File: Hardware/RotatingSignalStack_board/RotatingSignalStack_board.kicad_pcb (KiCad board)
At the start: 2 copper layers, 69.1 x 69 mm, 32 parts, among them J1 8P8C_LED_Shielded, J2 Conn_01x05_Pin, SW1 SW_Push, SW2 SW_Push, U1 OKI, U3 Teensy4.1_DEV-16771

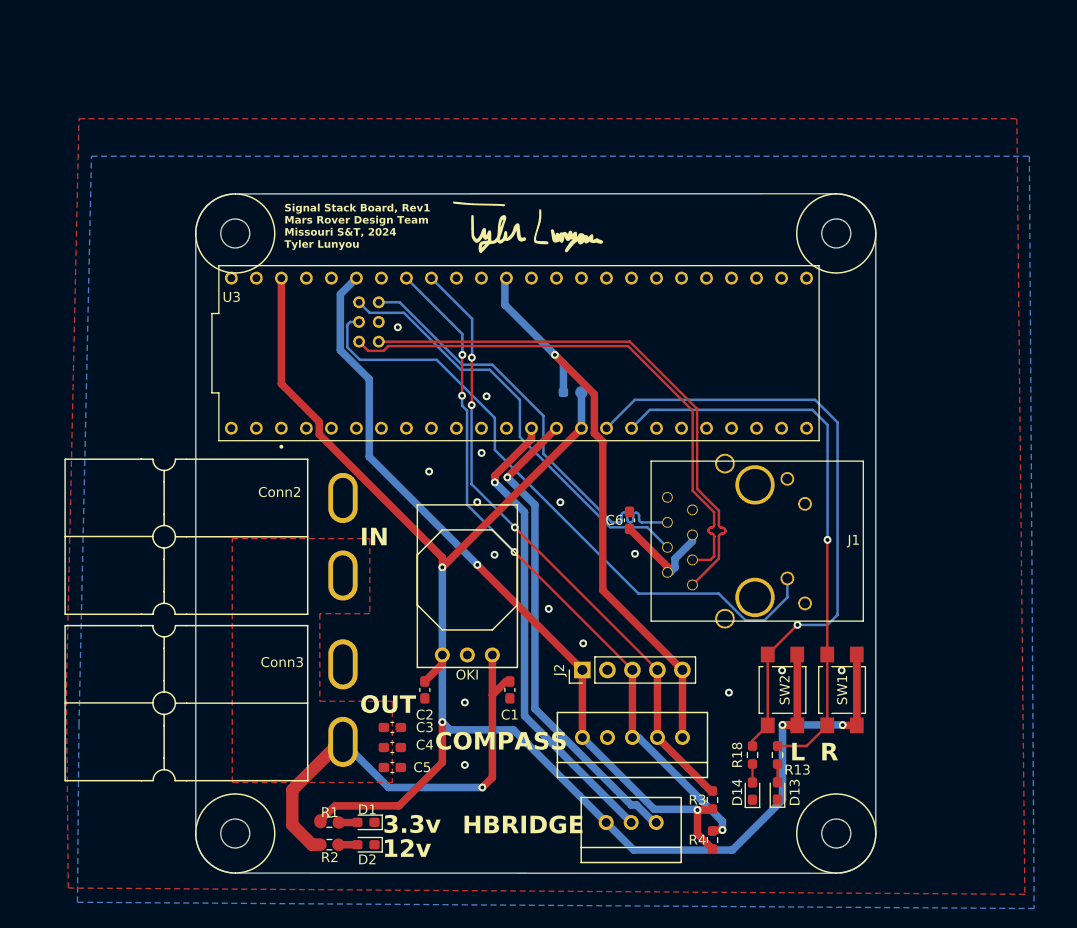
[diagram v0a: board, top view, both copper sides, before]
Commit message: Redid layout
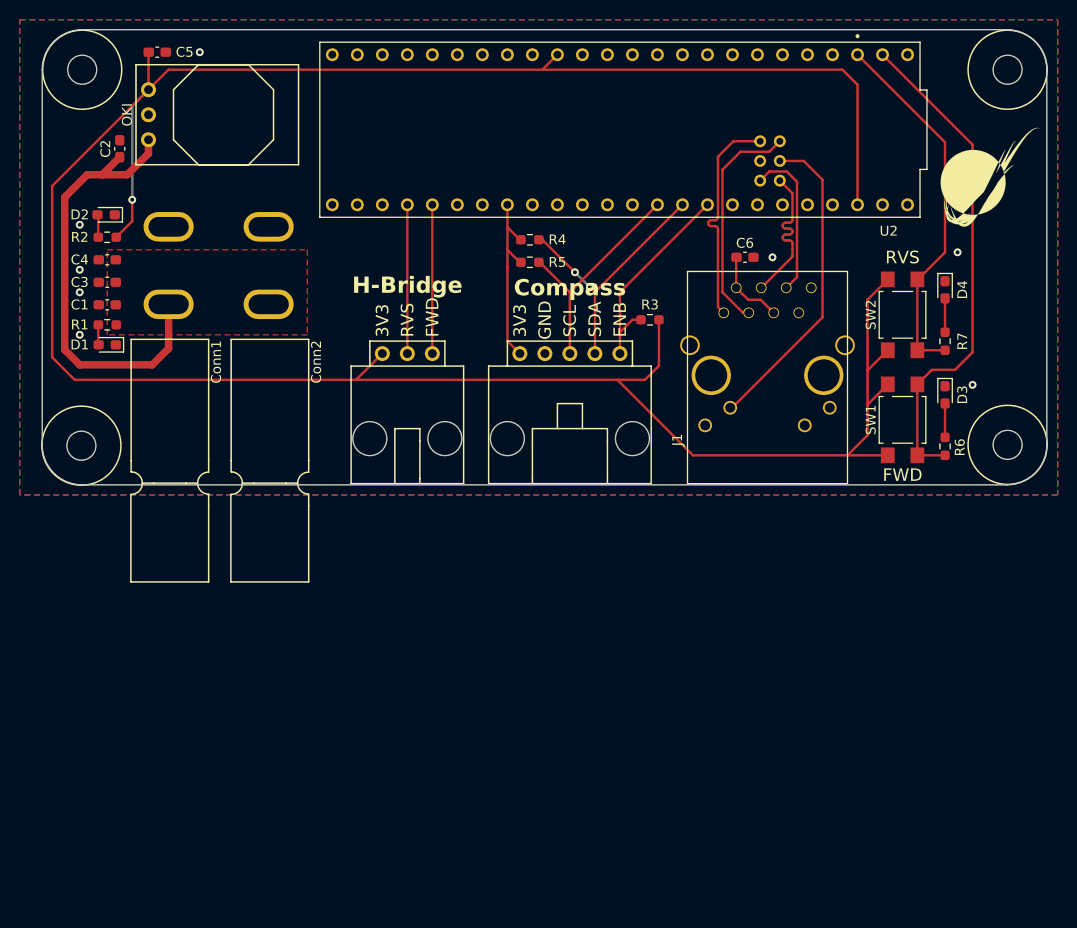
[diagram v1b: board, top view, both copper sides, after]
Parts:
- removed Conn6: Molex_SL_05, MRDT_Connectors:MOLEX_SL_05_Vertical
- removed D13, D14: Blue, LED_SMD:LED_0603_1608Metric_Pad1.05x0.95mm_HandSolder
- removed the G*** at (151.2, 87.1)
- removed J2: Conn_01x05_Pin, Connector_PinHeader_2.54mm:PinHeader_1x05_P2.54mm_Vertical
- removed R13, R18: 100, Resistor_SMD:R_0603_1608Metric_Pad0.98x0.95mm_HandSolder
- removed U3: Teensy4.1_DEV-16771, MRDT_Shields:Teensy_4_1_Ethernet
- added Conn4: Molex_SL_03, MRDT_Connectors:MOLEX_SL_03_Horizontal, F.Cu at (136.7, 99.9)
- added D3: Blue, LED_SMD:LED_0603_1608Metric_Pad1.05x0.95mm_HandSolder, F.Cu at (188.7, 104.1)
- added D4: Blue, LED_SMD:LED_0603_1608Metric_Pad1.05x0.95mm_HandSolder, F.Cu at (188.7, 93.5)
- added G***: LOGO, MRDT_Silkscreens:0_MRDT_Logo_10mm, F.Cu at (193.3, 82.0)
- added G***: LOGO, MRDT_Silkscreens:z_sig_Grant_Brinker_25mmx6, B.Cu at (180.3, 74.9)
- added G***: LOGO, MRDT_Silkscreens:yagi, B.Cu at (133.9, 89.4)
- added G***: LOGO, MRDT_Silkscreens:0_MRDT_Logo_10mm, B.Cu at (128.3, 77.5)
- added R6: 100, Resistor_SMD:R_0603_1608Metric_Pad0.98x0.95mm_HandSolder, F.Cu at (188.7, 109.4)
- added R7: 100, Resistor_SMD:R_0603_1608Metric_Pad0.98x0.95mm_HandSolder, F.Cu at (188.7, 98.7)
- added U2: Teensy4.1_DEV-16771, MRDT_Shields:Teensy_4_1_Ethernet, F.Cu at (155.7, 77.2)
- C1: value 10uF -> 0.1uF
- C3: value 0.1uF -> 10uF
- C4: value 10uF -> 22uF
- C5: value 22uF -> 10uF
- Conn1: value Molex_SL_03 -> AndersonPP; footprint MRDT_Connectors:MOLEX_SL_03_Vertical -> MRDT_Connectors:Square_Anderson_2_H_Stacked
- Conn2: footprint MRDT_Connectors:Square_Anderson_2_H_Side_By_Side -> MRDT_Connectors:Square_Anderson_2_H_Stacked
- Conn3: value AndersonPP -> Molex_SL_05; footprint MRDT_Connectors:Square_Anderson_2_H_Side_By_Side -> MRDT_Connectors:MOLEX_SL_05_Horizontal
- R1: value 100 -> 1k
- R2: value 1k -> 100
- R3: value 4.7k -> 0
- R5: value 0 -> 4.7k; moved to F.Cu
- moved V3 97.7 mm to (105.1, 75.1), turned to 90 degrees
- moved C5 76.5 mm to (108.7, 69.3)
- moved Conn1 73.1 mm to (108.9, 94.6), turned to 90 degrees
- moved V2 72.4 mm to (191.1, 75.1), turned to 0 degrees
- moved D2 69.2 mm to (103.5, 85.9)
- moved R2 65.7 mm to (103.6, 88.1)
- moved R4 63.7 mm to (146.6, 88.4), turned to 0 degrees
- moved C2 63.1 mm to (104.9, 79.1), turned to 90 degrees
- moved U1 62.9 mm to (107.8, 78.2), turned to 90 degrees
- moved C4 57.4 mm to (103.6, 90.4), turned to 180 degrees
- moved C1 56.6 mm to (103.6, 95.0), turned to 180 degrees
- moved R1 55.3 mm to (103.6, 97.0)
- moved D1 55.2 mm to (103.6, 99.1)
- moved C3 53.7 mm to (103.6, 92.7), turned to 180 degrees
- moved R3 49.2 mm to (158.8, 96.5), turned to 180 degrees
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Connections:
- C2 pad 1: +3.3V -> +12V
- C5 pad 1: +12V -> +3.3V
- Conn1 pad 1: HB_FWD -> GND
- Conn3 pad 1: GND -> MAG ENABLE
- Conn3 pad 2: +12V -> I2C SDA
- R1 pad 1: +3.3V -> Net-(D1-A)
- R1 pad 2: Net-(D1-A) -> +12V
- R2 pad 1: Net-(D2-A) -> +3.3V
- R2 pad 2: +12V -> Net-(D2-A)
- R3 pad 1: COMP PWR -> +3.3V
- R3 pad 2: I2C SDA -> MAG ENABLE
- R4 pad 2: I2C SCL -> I2C SDA
- R5 pad 1: +3.3V -> COMP PWR
- R5 pad 2: MAG ENABLE -> I2C SCL
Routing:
- net +3.3V: track 171.2 -> 266.8 mm, vias 4 -> 1
- net COMP PWR: track 78.4 -> 19.4 mm, vias 2 -> 0
- net I2C SCL: track 70.8 -> 23.2 mm, vias 4 -> 0
- net I2C SDA: track 64.0 -> 26.7 mm, vias 3 -> 2
- net MAG ENABLE: track 58.4 -> 21.5 mm, vias 1 -> 0
- net HB_FWD: track 48.8 -> 15.1 mm, vias 1 -> 0
- net /Tx+: track 55.8 -> 22.5 mm
- net /Tx-: track 55.8 -> 23.0 mm
- net /LED: track 64.6 -> 32.3 mm
- net HB_RVS: track 47.3 -> 15.1 mm, vias 1 -> 0
- net /Rx+: track 43.8 -> 15.6 mm
- net /Rx-: track 43.7 -> 15.8 mm
- net JOG B: track 63.8 -> 37.7 mm, vias 1 -> 0
- net JOG A: track 57.8 -> 51.0 mm, vias 1 -> 0
- net Net-(D4-A): track 0.00 -> 3.44 mm
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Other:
- board size 69.1 x 69 mm -> 102 x 46.2 mm
- board text added: "3V3"
- board text added: "Compass"
- board text added: "ENB"
- board text added: "FWD"
- board text added: "GND"
- board text added: "H-Bridge"
- board text added: "RVS"
- board text added: "SCL"
- board text added: "SDA"
- board text added: "Signal Stack Board, Rev1 Mars Rover Design Team Missouri S&T, 2024 Grant Brinker"
- board text removed: "12v"
- board text removed: "3.3v"
- board text removed: "3.3v Direct Power Compass"
- board text removed: "COMPASS"
- board text removed: "HBRIDGE"
- board text removed: "IN"
- board text removed: "L"
- board text removed: "OUT"
- board text removed: "R"
- board text removed: "Signal Stack Board, Rev1 Mars Rover Design Team Missouri S&T, 2024 Tyler Lunyou"
